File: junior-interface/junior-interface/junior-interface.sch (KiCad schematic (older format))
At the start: 19 parts, among them IC13 74LS27, IC14 74LS01, IC15 74LS30, IC16 74LS00, IC17 GAL16V8, IC2 2114, IC3 2114, IC4 2716, IC5 2716, J12 Conn_01x03_Male

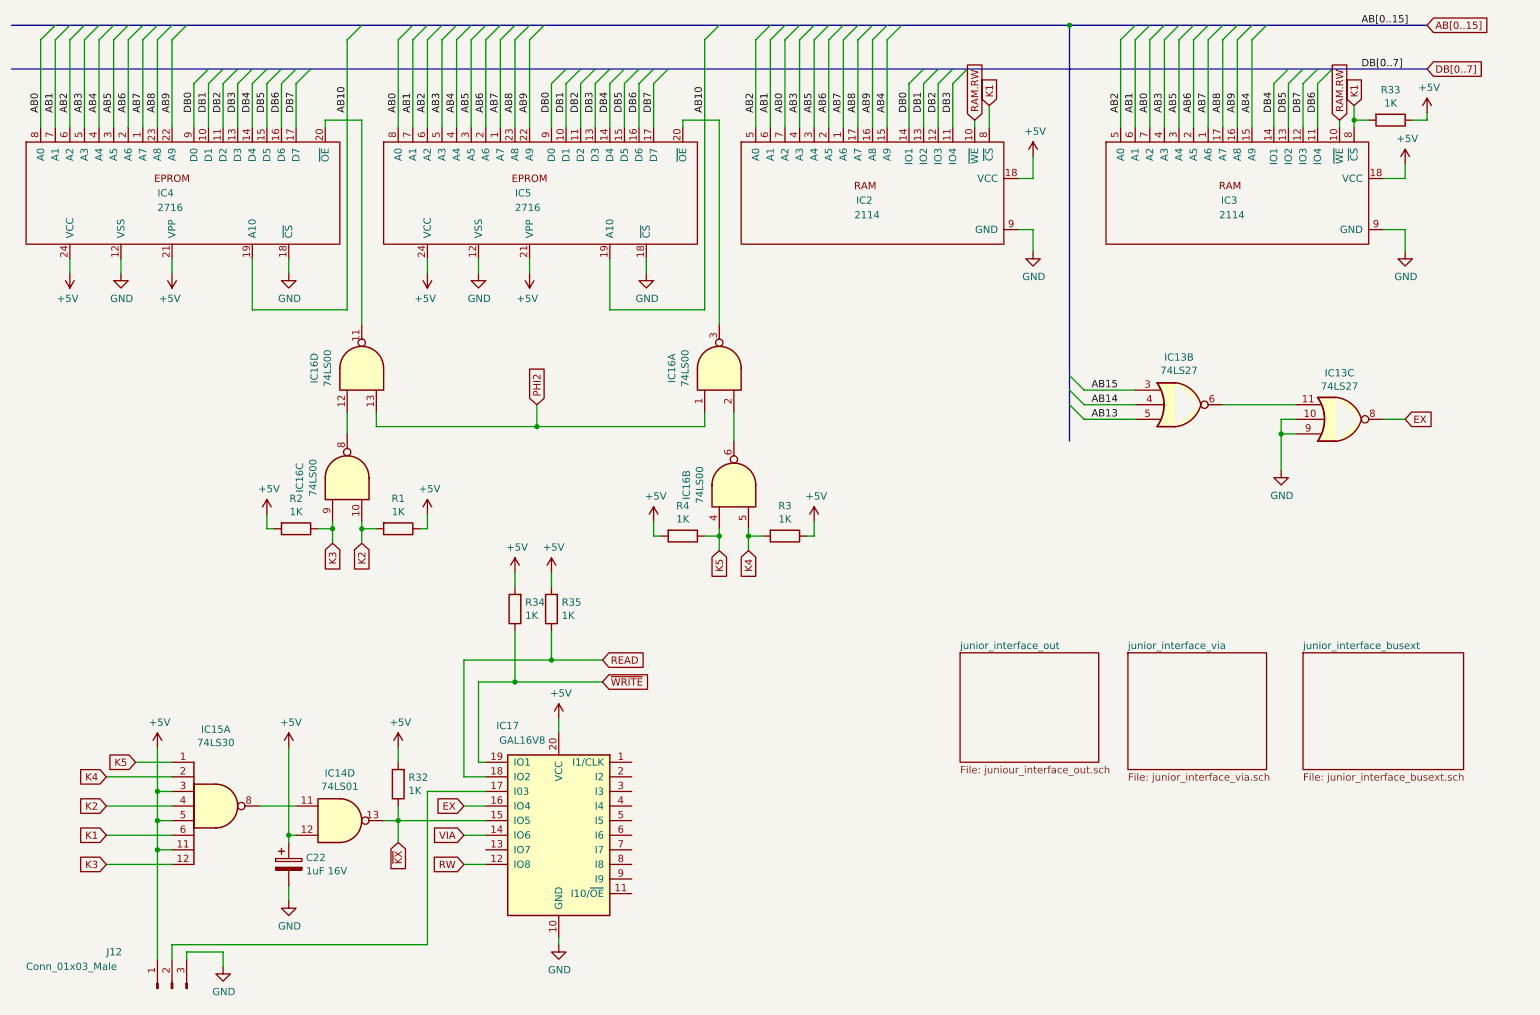
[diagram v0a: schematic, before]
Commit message: junior interface modifs
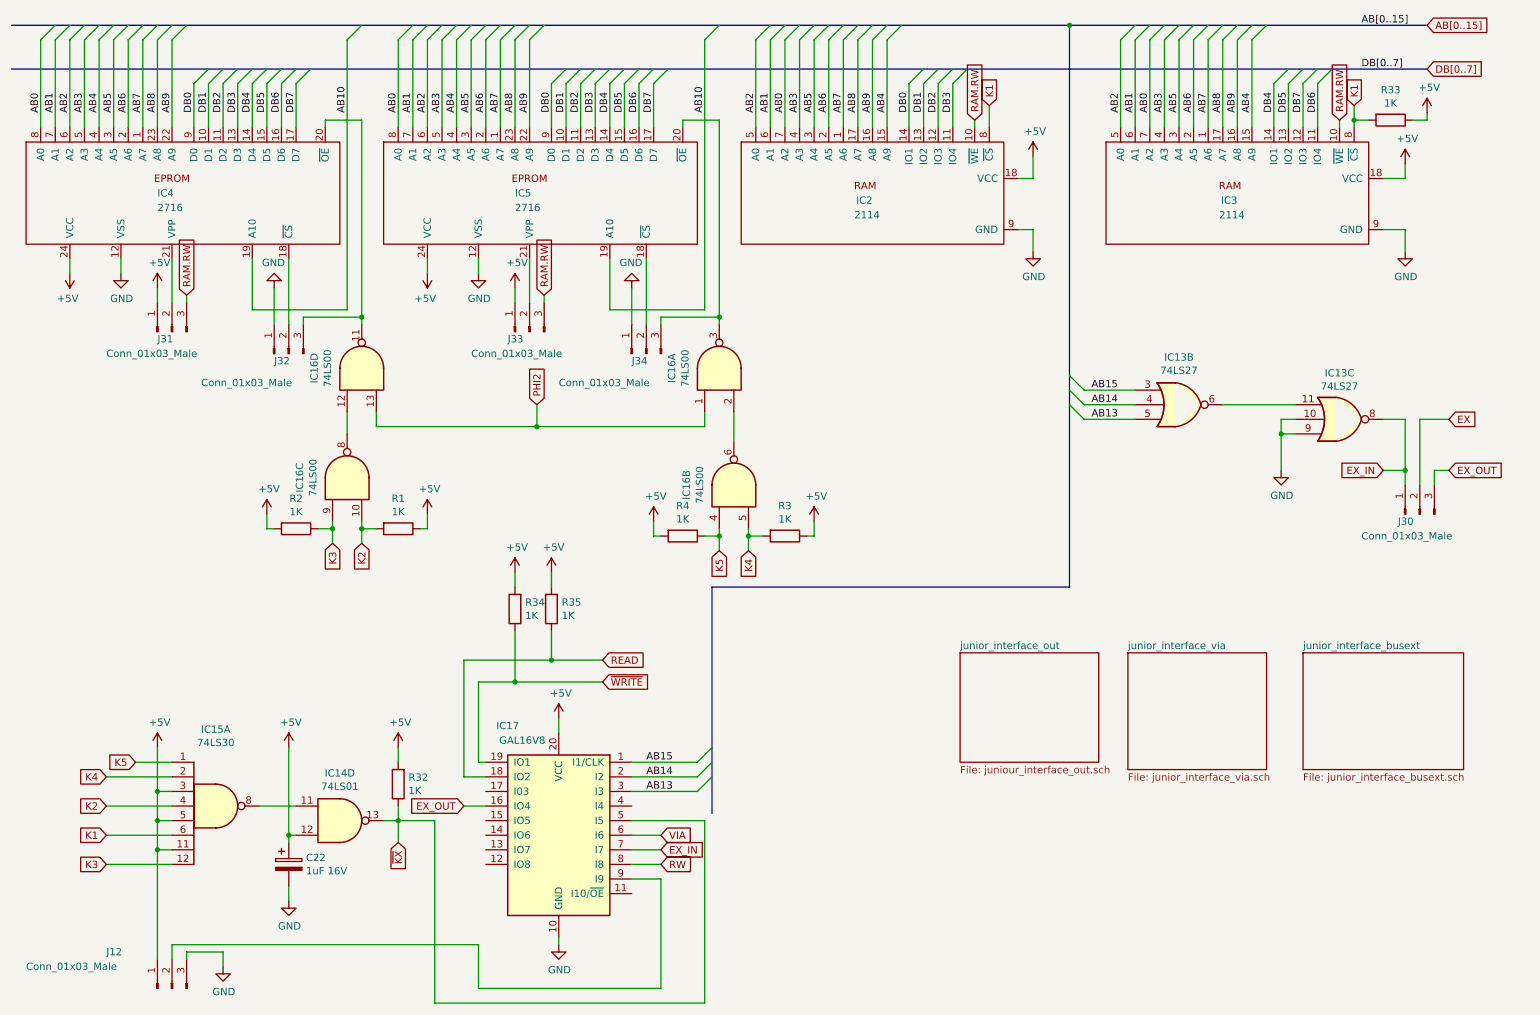
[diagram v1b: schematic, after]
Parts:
- added J30, J31, J32, J33, J34: Conn_01x03_Male, Pin_Headers:Pin_Header_Straight_1x03_Pitch2.54mm, symbol Connector:Conn_01x03_Male
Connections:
- net +5V: now also J31.1 (Pin_1), J33.1 (Pin_1); no longer IC4.21 (VPP), IC5.21 (VPP)
- net AB13: now also IC17.3 (I3)
- net AB14: now also IC17.2 (I2)
- net AB15: now also IC17.1 (I1/CLK)
- net EX: now also J30.2 (Pin_2); no longer IC13.8, IC17.16 (IO4)
- net GND: now also J32.1 (Pin_1), J34.1 (Pin_1); no longer IC4.18 (~CS~), IC5.18 (~CS~)
- net RAM.RW: now also J31.3 (Pin_3), J33.3 (Pin_3)
- net RW: now also IC17.8 (I8); no longer IC17.12 (IO8)
- net VIA: now also IC17.6 (I6); no longer IC17.14 (IO6)
- net ~KX~: now also IC17.5 (I5); no longer IC17.15 (IO5)
- net at IC16.11, IC4.20 (~OE~): now also J32.3 (Pin_3)
- net at IC16.3, IC5.20 (~OE~): now also J34.3 (Pin_3)
- net at IC17.17 (I03): no longer J12.2 (Pin_2)
- net EX_IN: now reaches IC17.7 (I7)
- net EX_IN: now also IC13.8, J30.1 (Pin_1)
- net at IC17.9 (I9): now also J12.2 (Pin_2)
- new net: IC4.18 (~CS~), J32.2 (Pin_2)
- new net: IC4.21 (VPP), J31.2 (Pin_2)
- new net: IC5.18 (~CS~), J34.2 (Pin_2)
- new net: IC5.21 (VPP), J33.2 (Pin_2)
- new net EX_OUT: IC17.16 (IO4), J30.3 (Pin_3)
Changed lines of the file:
@@
 L power:GND #PWR0113
 U 1 1 5FACA129
-P 5150 2550
-F 0 "#PWR0113" H 5150 2300 50  0001 C CNN
-F 1 "GND" H 5155 2377 50  0000 C CNN
-F 2 "" H 5150 2550 50  0001 C CNN
-F 3 "" H 5150 2550 50  0001 C CNN
-	1    5150 2550
-	1    0    0    -1
+P 5050 2650
+F 0 "#PWR0113" H 5050 2400 50  0001 C CNN
+F 1 "GND" H 5055 2477 50  0000 C CNN
+F 2 "" H 5050 2650 50  0001 C CNN
+F 3 "" H 5050 2650 50  0001 C CNN
+	1    5050 2650
+	-1   0    0    1
 $EndComp
 $Comp
 L power:GND #PWR0114
 U 1 1 5FACA3B0
-P 2700 2550
-F 0 "#PWR0114" H 2700 2300 50  0001 C CNN
-F 1 "GND" H 2705 2377 50  0000 C CNN
-F 2 "" H 2700 2550 50  0001 C CNN
-F 3 "" H 2700 2550 50  0001 C CNN
-	1    2700 2550
-	1    0    0    -1
-$EndComp
-Wire Wire Line
-	5150 2450 5150 2550
-Wire Wire Line
-	2700 2450 2700 2550
-$Comp
-L power:+5V #PWR0115
-U 1 1 5FAD1823
-P 4350 2550
-F 0 "#PWR0115" H 4350 2400 50  0001 C CNN
-F 1 "+5V" H 4365 2723 50  0000 C CNN
-F 2 "" H 4350 2550 50  0001 C CNN
-F 3 "" H 4350 2550 50  0001 C CNN
-	1    4350 2550
+P 2600 2650
+F 0 "#PWR0114" H 2600 2400 50  0001 C CNN
+F 1 "GND" H 2605 2477 50  0000 C CNN
+F 2 "" H 2600 2650 50  0001 C CNN
+F 3 "" H 2600 2650 50  0001 C CNN
+	1    2600 2650
 	-1   0    0    1
 $EndComp
@@
 L power:+5V #PWR0116
 U 1 1 5FAD1ADF
-P 1900 2550
-F 0 "#PWR0116" H 1900 2400 50  0001 C CNN
-F 1 "+5V" H 1915 2723 50  0000 C CNN
-F 2 "" H 1900 2550 50  0001 C CNN
-F 3 "" H 1900 2550 50  0001 C CNN
-	1    1900 2550
-	-1   0    0    1
+P 1800 2650
+F 0 "#PWR0116" H 1800 2500 50  0001 C CNN
+F 1 "+5V" H 1815 2823 50  0000 C CNN
+F 2 "" H 1800 2650 50  0001 C CNN
+F 3 "" H 1800 2650 50  0001 C CNN
+	1    1800 2650
+	1    0    0    -1
 $EndComp
 $Comp
@@
 	1550 2450 1550 2550
 Wire Wire Line
-	1900 2450 1900 2550
-Wire Wire Line
 	3650 2450 3650 2550
 Wire Wire Line
 	4000 2450 4000 2550
-Wire Wire Line
-	4350 2450 4350 2550
 $Comp
 L power:GND #PWR0121
@@
 	2950 1500 3200 1500
 Wire Wire Line
-	3200 1500 3200 2900
+	3200 1500 3200 2850
 Wire Wire Line
 	5400 1550 5400 1500
@@
 	5400 1500 5650 1500
 Wire Wire Line
-	5650 1500 5650 2900
+	5650 1500 5650 2850
 Text Label 3550 1450 1    50   ~ 0
 AB1
@@
 Text Label 8200 3550 0    50   ~ 0
 AB13
-Text GLabel 10350 3550 2    50   Input ~ 0
+Text GLabel 10650 3550 2    50   Input ~ 0
 EX
-Wire Wire Line
-	10350 3550 10200 3550
 Text GLabel 1650 5900 0    50   Input ~ 0
 K5
@@
 Wire Wire Line
 	4550 7100 4550 7150
-Text GLabel 3900 6200 0    50   Input ~ 0
-EX
-Wire Wire Line
-	3900 6200 4050 6200
-Text GLabel 3900 6400 0    50   Input ~ 0
+Text GLabel 5250 6500 2    50   Input ~ 0
+EX_IN
+Text GLabel 5250 6400 2    50   Input ~ 0
 VIA
-Wire Wire Line
-	3900 6400 4050 6400
-Text GLabel 3900 6600 0    50   Input ~ 0
+Text GLabel 5250 6600 2    50   Input ~ 0
 RW
 $Comp
@@
 Wire Wire Line
 	1900 7250 1900 7150
-Wire Wire Line
-	1900 7150 3650 7150
-Wire Wire Line
-	3650 7150 3650 6100
-Wire Wire Line
-	3650 6100 4050 6100
 $Comp
 L power:GND #PWR0140
@@
 Connection ~ 4500 5200
 Wire Wire Line
-	3450 6300 4050 6300
-Wire Wire Line
-	3900 6600 4050 6600
+	3450 6300 3700 6300
 Wire Bus Line
-	8050 850  8050 3700
+	8050 4700 5600 4700
+Entry Wire Line
+	5500 5900 5600 5800
+Entry Wire Line
+	5500 6000 5600 5900
+Entry Wire Line
+	5500 6100 5600 6000
+Wire Wire Line
+	5500 5900 5050 5900
+Wire Wire Line
+	5050 6000 5500 6000
+Wire Wire Line
+	5500 6100 5050 6100
+Text Label 5150 5900 0    50   ~ 0
+AB15
+Text Label 5150 6000 0    50   ~ 0
+AB14
+Text Label 5150 6100 0    50   ~ 0
+AB13
+$Comp
+L Connector:Conn_01x03_Male J31
+U 1 1 5FC20CB9
+P 1900 2950
+F 0 "J31" V 1850 3050 50  0000 R CNN
+F 1 "Conn_01x03_Male" V 1750 3400 50  0000 R CNN
+F 2 "Pin_Headers:Pin_Header_Straight_1x03_Pitch2.54mm" H 1900 2950 50  0001 C CNN
+F 3 "~" H 1900 2950 50  0001 C CNN
+	1    1900 2950
+	0    -1   -1   0
+$EndComp
+Wire Wire Line
+	1900 2450 1900 2750
+Wire Wire Line
+	1800 2650 1800 2750
+Text GLabel 2000 2700 1    50   Input ~ 0
+RAM.RW
+Wire Wire Line
+	2000 2700 2000 2750
+$Comp
+L power:+5V #PWR0115
+U 1 1 5FC58807
+P 4250 2650
+F 0 "#PWR0115" H 4250 2500 50  0001 C CNN
+F 1 "+5V" H 4265 2823 50  0000 C CNN
+F 2 "" H 4250 2650 50  0001 C CNN
+F 3 "" H 4250 2650 50  0001 C CNN
+	1    4250 2650
+	1    0    0    -1
+$EndComp
+$Comp
+L Connector:Conn_01x03_Male J33
+U 1 1 5FC58811
+P 4350 2950
+F 0 "J33" V 4300 3100 50  0000 R CNN
+F 1 "Conn_01x03_Male" V 4200 3350 50  0000 R CNN
+F 2 "Pin_Headers:Pin_Header_Straight_1x03_Pitch2.54mm" H 4350 2950 50  0001 C CNN
+F 3 "~" H 4350 2950 50  0001 C CNN
+	1    4350 2950
+	0    -1   -1   0
+$EndComp
+Wire Wire Line
+	4350 2450 4350 2750
+Wire Wire Line
+	4250 2650 4250 2750
+Text GLabel 4450 2700 1    50   Input ~ 0
+RAM.RW
+Wire Wire Line
+	4450 2700 4450 2750
+$Comp
+L Connector:Conn_01x03_Male J32
+U 1 1 5FC6786F
+P 2700 3100
+F 0 "J32" V 2650 3200 50  0000 R CNN
+F 1 "Conn_01x03_Male" V 2500 3700 50  0000 R CNN
+F 2 "Pin_Headers:Pin_Header_Straight_1x03_Pitch2.54mm" H 2700 3100 50  0001 C CNN
+F 3 "~" H 2700 3100 50  0001 C CNN
+	1    2700 3100
+	0    -1   -1   0
+$EndComp
+Wire Wire Line
+	2600 2650 2600 2900
+Wire Wire Line
+	2700 2450 2700 2900
+Wire Wire Line
+	2800 2900 2800 2850
+Wire Wire Line
+	2800 2850 3200 2850
+Connection ~ 3200 2850
+Wire Wire Line
+	3200 2850 3200 2900
+$Comp
+L Connector:Conn_01x03_Male J34
+U 1 1 5FC933A1
+P 5150 3100
+F 0 "J34" V 5100 3200 50  0000 R CNN
+F 1 "Conn_01x03_Male" V 4950 3700 50  0000 R CNN
+F 2 "Pin_Headers:Pin_Header_Straight_1x03_Pitch2.54mm" H 5150 3100 50  0001 C CNN
+F 3 "~" H 5150 3100 50  0001 C CNN
+	1    5150 3100
+	0    -1   -1   0
+$EndComp
+Wire Wire Line
+	5250 2900 5250 2850
+Wire Wire Line
+	5250 2850 5650 2850
+Connection ~ 5650 2850
+Wire Wire Line
+	5650 2850 5650 2900
+Wire Wire Line
+	5050 2650 5050 2900
+Wire Wire Line
+	5150 2450 5150 2900
+Wire Wire Line
+	5550 7550 3700 7550
+Wire Wire Line
+	3700 7550 3700 6300
+Wire Wire Line
+	4000 7150 4000 7450
+Wire Wire Line
+	4000 7450 5250 7450
+Wire Wire Line
+	5250 7450 5250 6700
+Wire Wire Line
+	5250 6700 5050 6700
+Wire Wire Line
+	1900 7150 4000 7150
+Wire Wire Line
+	5050 6500 5250 6500
+Wire Wire Line
+	5250 6600 5050 6600
+Wire Wire Line
+	5050 6300 5550 6300
+Wire Wire Line
+	5550 6300 5550 7550
+Wire Wire Line
+	5250 6400 5050 6400
+Text GLabel 3900 6200 0    50   Input ~ 0
+EX_OUT
+Wire Wire Line
+	3900 6200 4050 6200
+$Comp
+L Connector:Conn_01x03_Male J30
+U 1 1 5FF3480A
+P 10450 4200
+F 0 "J30" V 10400 4350 50  0000 R CNN
+F 1 "Conn_01x03_Male" V 10300 4600 50  0000 R CNN
+F 2 "Pin_Headers:Pin_Header_Straight_1x03_Pitch2.54mm" H 10450 4200 50  0001 C CNN
+F 3 "~" H 10450 4200 50  0001 C CNN
+	1    10450 4200
+	0    -1   -1   0
+$EndComp
+Wire Wire Line
+	10650 3550 10450 3550
+Wire Wire Line
+	10450 3550 10450 4000
+Wire Wire Line
+	10200 3550 10350 3550
+Wire Wire Line
+	10350 3550 10350 3900
+Text GLabel 10650 3900 2    50   Input ~ 0
+EX_OUT
+Text GLabel 10200 3900 0    50   Input ~ 0
+EX_IN
+Wire Wire Line
+	10200 3900 10350 3900
+Connection ~ 10350 3900
+Wire Wire Line
+	10350 3900 10350 4000
+Wire Wire Line
+	10650 3900 10550 3900
+Wire Wire Line
+	10550 3900 10550 4000
+Wire Bus Line
+	5600 4700 5600 6250
+Wire Bus Line
+	8050 850  8050 4700
 Wire Bus Line
 	8050 850  10500 850

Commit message: junior bus
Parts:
- J12, J30, J31, J32, J33, J34: footprint Pin_Headers:Pin_Header_Straight_1x03_Pitch2.54mm -> elektor:CONN-3
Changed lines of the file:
@@
 F 0 "J12" V 2150 7900 50  0000 R CNN
 F 1 "Conn_01x03_Male" V 2050 8450 50  0000 R CNN
-F 2 "Pin_Headers:Pin_Header_Straight_1x03_Pitch2.54mm" H 1900 7450 50  0001 C CNN
+F 2 "elektor:CONN-3" H 1900 7450 50  0001 C CNN
 F 3 "~" H 1900 7450 50  0001 C CNN
 	1    1900 7450
@@
 F 0 "J31" V 1850 3050 50  0000 R CNN
 F 1 "Conn_01x03_Male" V 1750 3400 50  0000 R CNN
-F 2 "Pin_Headers:Pin_Header_Straight_1x03_Pitch2.54mm" H 1900 2950 50  0001 C CNN
+F 2 "elektor:CONN-3" H 1900 2950 50  0001 C CNN
 F 3 "~" H 1900 2950 50  0001 C CNN
 	1    1900 2950
@@
 F 0 "J33" V 4300 3100 50  0000 R CNN
 F 1 "Conn_01x03_Male" V 4200 3350 50  0000 R CNN
-F 2 "Pin_Headers:Pin_Header_Straight_1x03_Pitch2.54mm" H 4350 2950 50  0001 C CNN
+F 2 "elektor:CONN-3" H 4350 2950 50  0001 C CNN
 F 3 "~" H 4350 2950 50  0001 C CNN
 	1    4350 2950
@@
 F 0 "J32" V 2650 3200 50  0000 R CNN
 F 1 "Conn_01x03_Male" V 2500 3700 50  0000 R CNN
-F 2 "Pin_Headers:Pin_Header_Straight_1x03_Pitch2.54mm" H 2700 3100 50  0001 C CNN
+F 2 "elektor:CONN-3" H 2700 3100 50  0001 C CNN
 F 3 "~" H 2700 3100 50  0001 C CNN
 	1    2700 3100
@@
 F 0 "J34" V 5100 3200 50  0000 R CNN
 F 1 "Conn_01x03_Male" V 4950 3700 50  0000 R CNN
-F 2 "Pin_Headers:Pin_Header_Straight_1x03_Pitch2.54mm" H 5150 3100 50  0001 C CNN
+F 2 "elektor:CONN-3" H 5150 3100 50  0001 C CNN
 F 3 "~" H 5150 3100 50  0001 C CNN
 	1    5150 3100
@@
 F 0 "J30" V 10400 4350 50  0000 R CNN
 F 1 "Conn_01x03_Male" V 10300 4600 50  0000 R CNN
-F 2 "Pin_Headers:Pin_Header_Straight_1x03_Pitch2.54mm" H 10450 4200 50  0001 C CNN
+F 2 "elektor:CONN-3" H 10450 4200 50  0001 C CNN
 F 3 "~" H 10450 4200 50  0001 C CNN
 	1    10450 4200
